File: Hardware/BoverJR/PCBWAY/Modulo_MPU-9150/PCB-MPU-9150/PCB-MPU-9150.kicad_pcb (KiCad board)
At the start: 2 copper layers, 15 x 20 mm, 16 parts, among them P1 CONN_01X08, U1 MPU-9150, U2 AP2112K-3.3

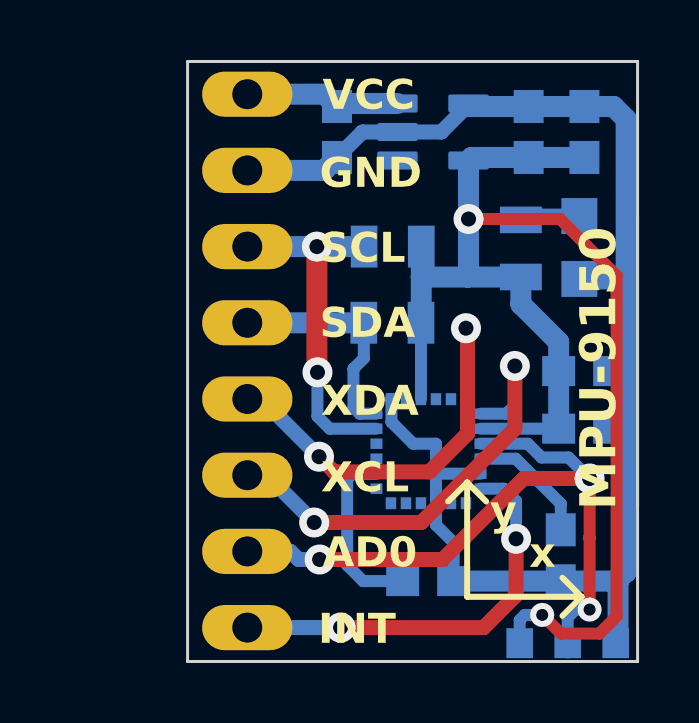
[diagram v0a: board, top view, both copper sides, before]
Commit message: realice algunos cambios en el pcb
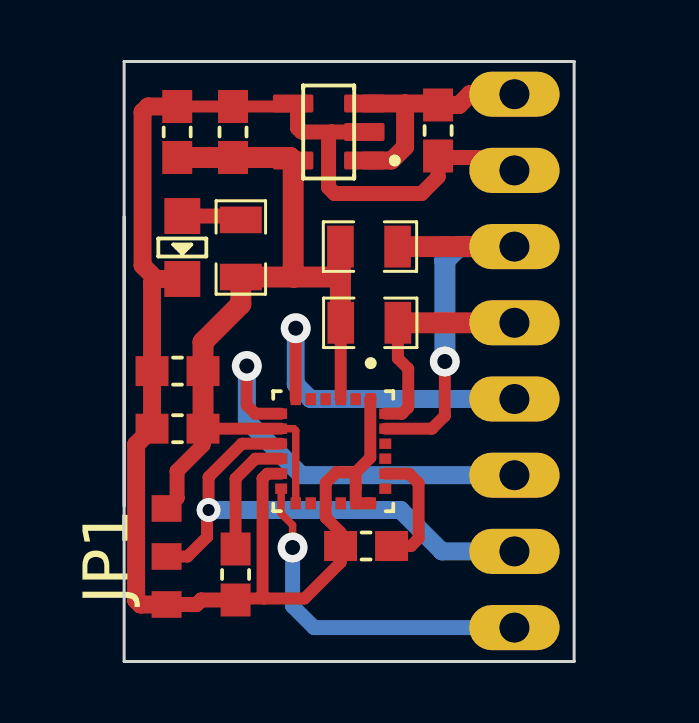
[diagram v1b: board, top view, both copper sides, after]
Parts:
- ?, P1: moved to B.Cu
- C1, C2, C3, C4, C5, C6, C7, JP1, LED1, R1, R2, R3, U1, U2: moved to F.Cu
- moved JP1 13.7 mm to (156.3, 56.5), turned to 90 degrees
- moved C5 13.6 mm to (156.7, 42.4)
- moved C3 13.6 mm to (156.7, 50.3), turned to 180 degrees
- moved C4 13.6 mm to (156.7, 52.2), turned to 180 degrees
- moved ? 13.4 mm to (156.8, 58.4), turned to 180 degrees
- moved LED1 13.2 mm to (156.8, 46.2)
- moved C2 10.9 mm to (158.6, 57.1)
- moved C6 9.85 mm to (158.5, 42.4)
- moved R3 9.33 mm to (158.8, 46.2)
- moved P1 8.91 mm to (167.9, 50.0), turned to 180 degrees
- moved U2 3.47 mm to (161.7, 42.4), turned to 180 degrees
- moved C7 3.37 mm to (165.3, 42.3)
- moved U1 3.17 mm to (161.9, 53.0)
- moved C1 2.38 mm to (162.9, 56.1), turned to 0 degrees
- moved R2 0.79 mm to (163.0, 46.2), turned to 0 degrees
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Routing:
- net +3.3V: track 46.0 -> 30.5 mm, vias 2 -> 0
- net GND: track 48.3 -> 55.3 mm
- net /AD0: track 22.8 -> 17.3 mm, vias 3 -> 1
- net /XDA: track 14.8 -> 11.7 mm, vias 2 -> 1
- net VCC: track 5.22 -> 8.17 mm
- net /INT: track 13.9 -> 11.8 mm, vias 2 -> 1
- net /SCL: track 11.7 -> 13.8 mm, vias 2 -> 1
- net Net-(U1-CPOUT): track 5.99 -> 4.09 mm
- net /XCL: track 16.4 -> 14.9 mm, vias 2 -> 1
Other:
- outline, holes or cut-outs redrawn
